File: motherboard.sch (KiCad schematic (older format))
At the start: 90 parts, among them P1 CONN_02X08, U1 STM32F411-LQFP64, U10 74LS125, U11 74LS125, U12 74LS125, U13 74LS125, U14 PCA9517A, U15 PCA9517A, U16 74LS125, U17 74LS125, U2 STM32F411-LQFP64, U3 AP7313, U4 74LS00, U5 74LS125, U6 FM25V20A-G, U7 FM25V20A-G, U8 FM25V20A-G, U9 FM25V20A-G, Y1 32k, Y2 8M(16pF), Y3 32k, Y4 8M(16pF)

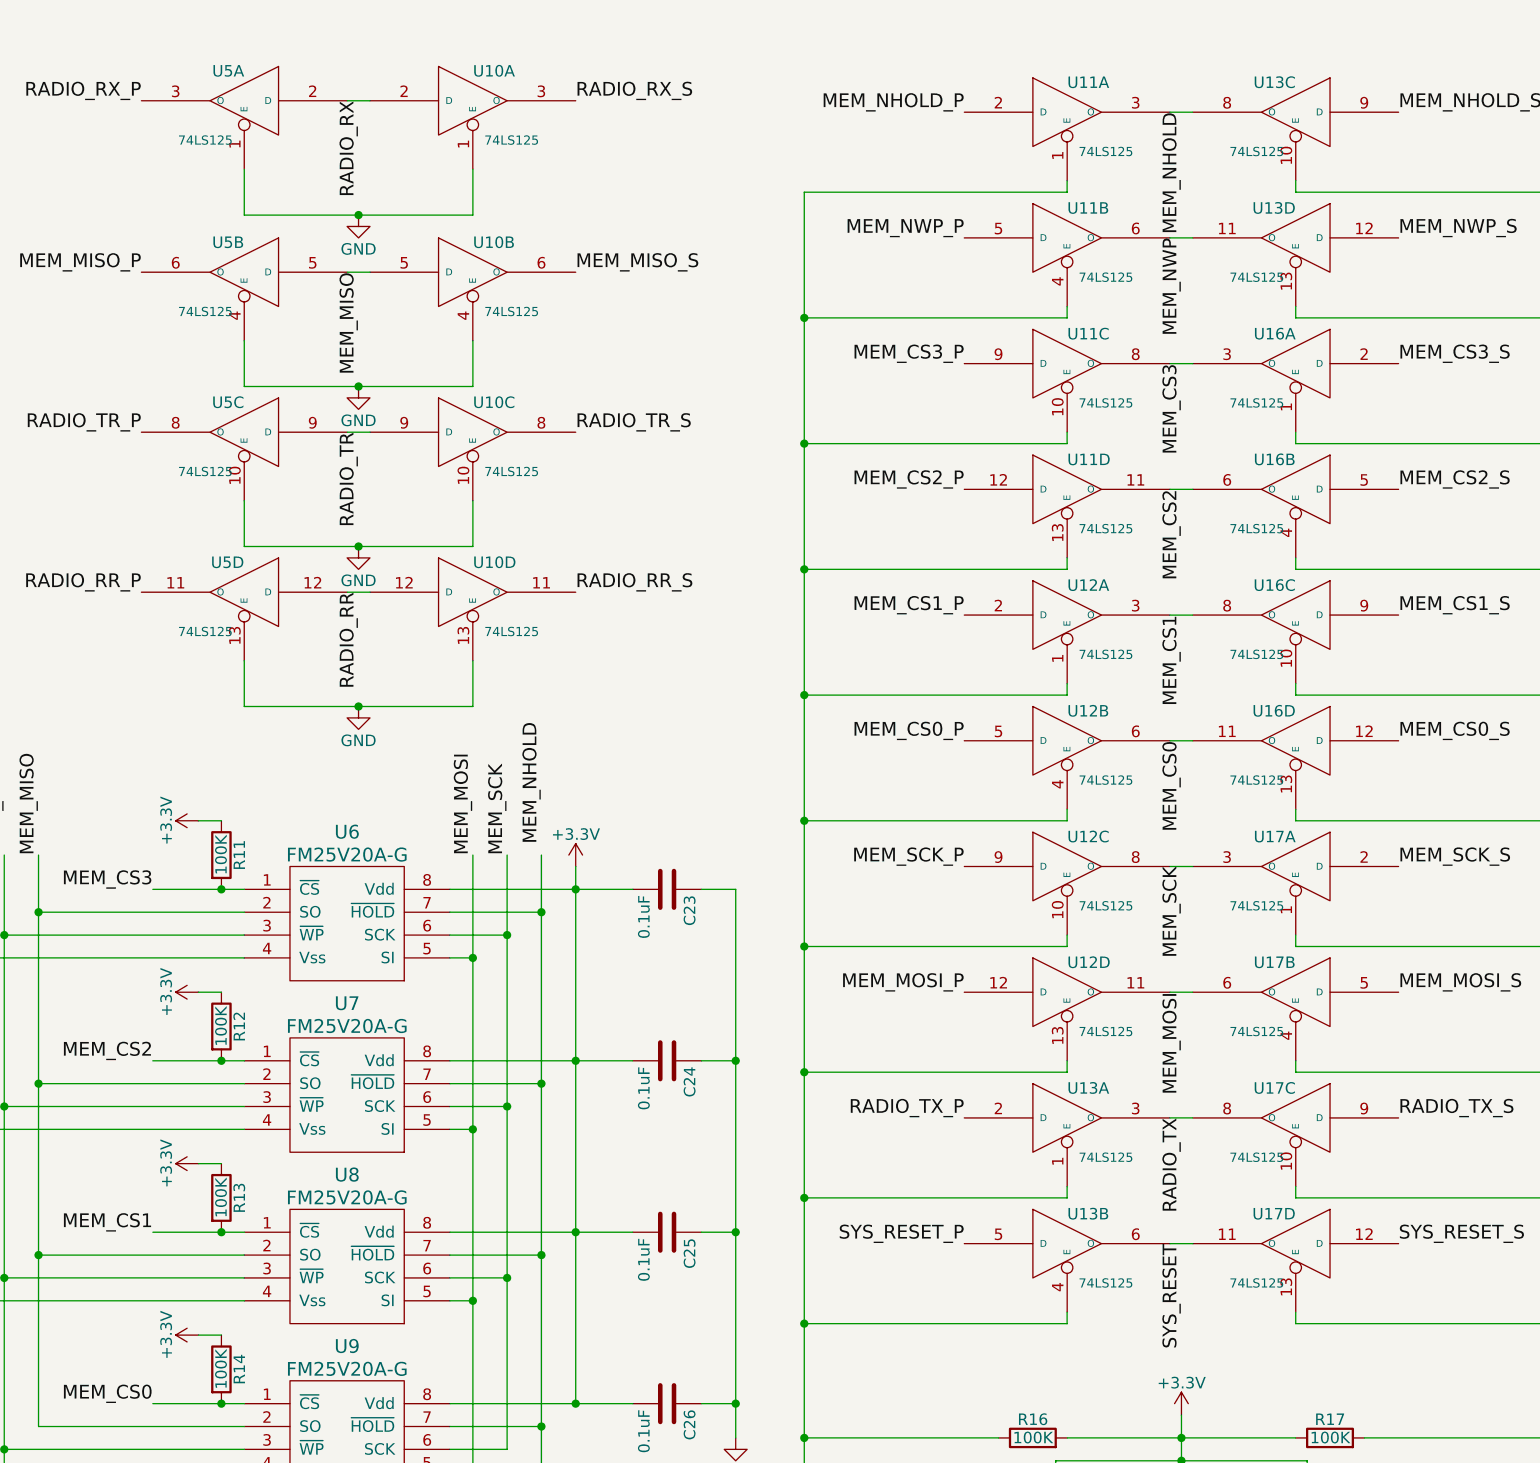
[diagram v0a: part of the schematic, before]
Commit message: Progress in laying out components
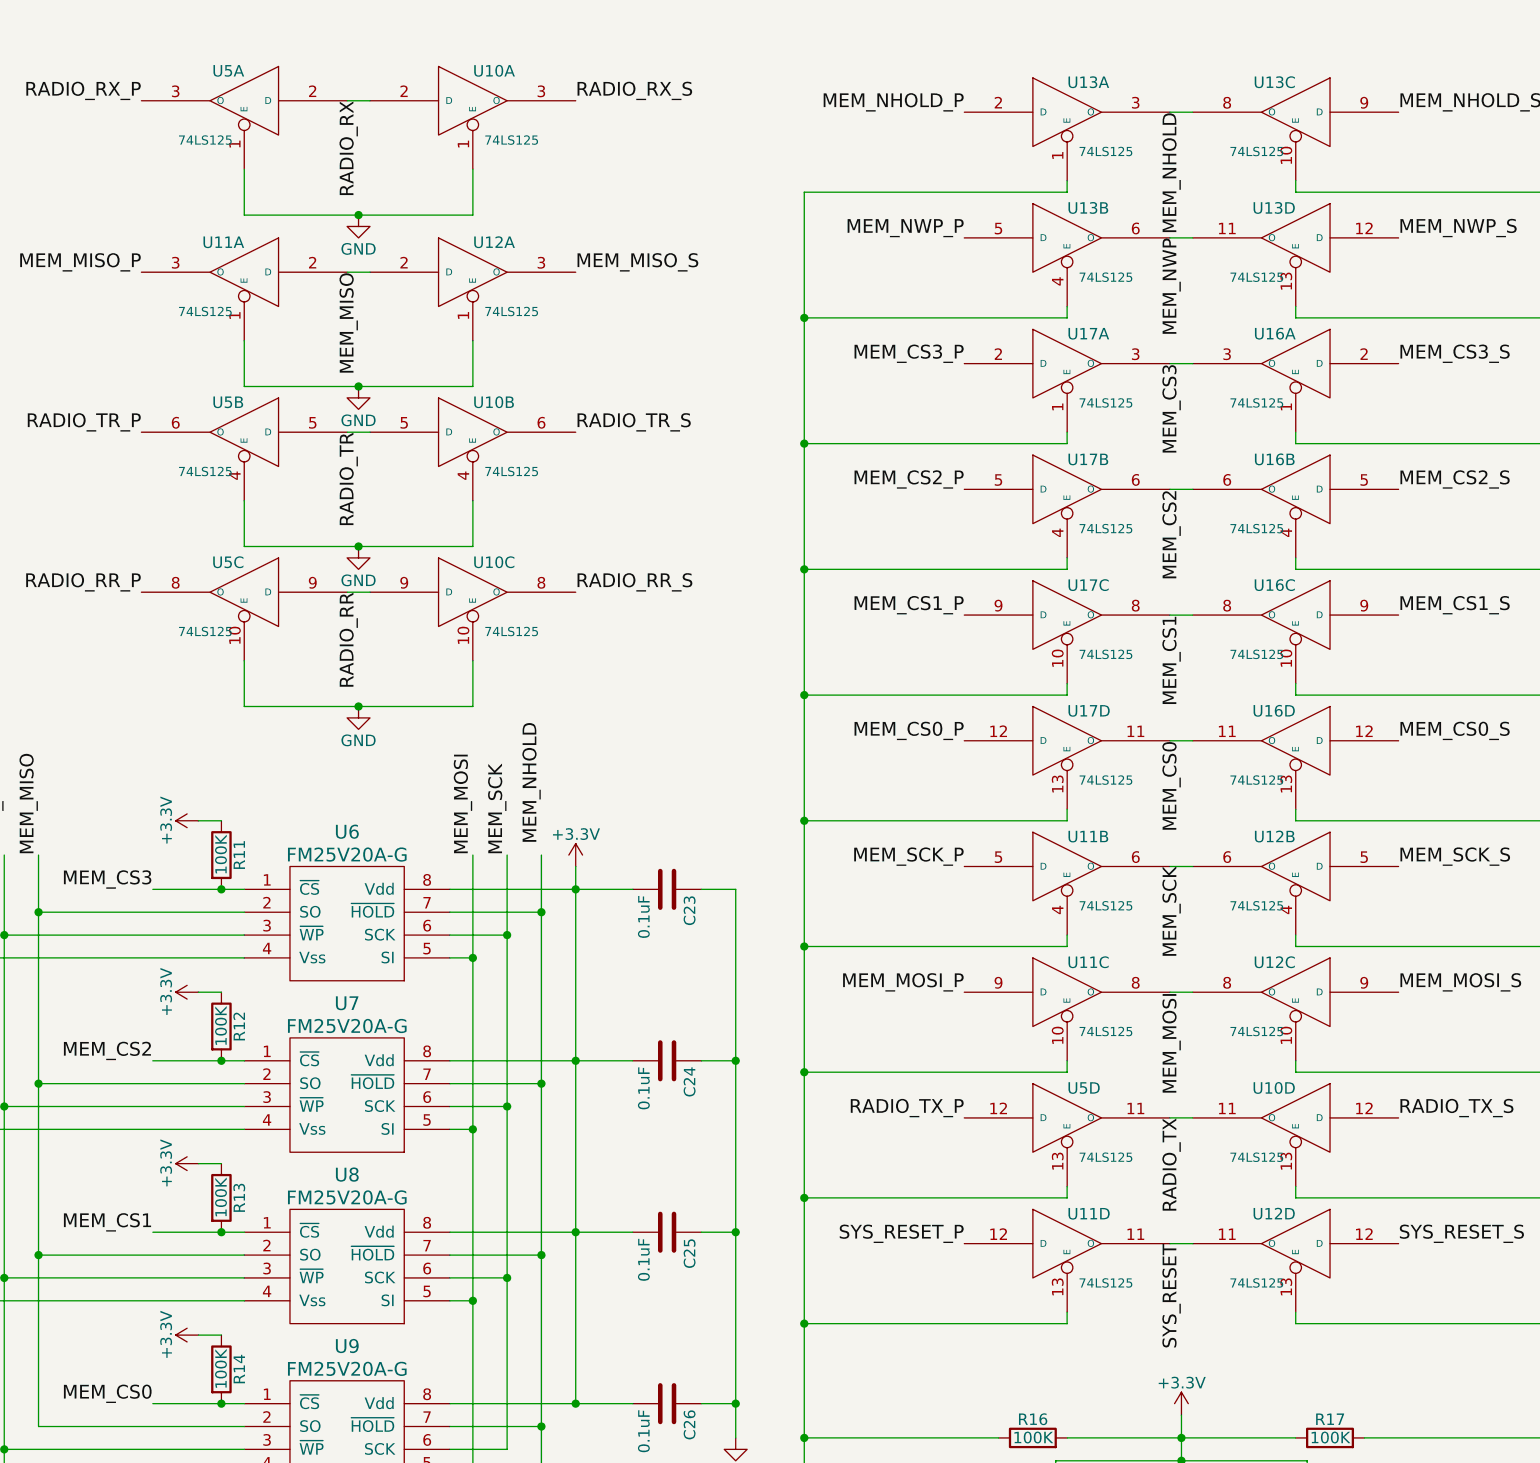
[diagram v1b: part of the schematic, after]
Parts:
- renumbered U17 to U10, U5 to U11, U12 to U11, U13 to U11, U10 to U12, U17 to U12, U11 to U13, U11 to U17, U12 to U17, U13 to U5
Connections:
- net GND: now also U10.10 (E), U10.4 (E), U11.1 (E), U12.1 (E), U5.10 (E), U5.4 (E); no longer U10.10 (E), U10.13 (E), U11.4 (E), U12.4 (E), U5.10 (E), U5.13 (E)
- net MEM_CS0: now also U17.11 (O); no longer U17.6 (O)
- net MEM_CS0_P: now also U17.12 (D); no longer U17.5 (D)
- net MEM_CS1: now also U17.8 (O); no longer U17.3 (O)
- net MEM_CS1_P: now also U17.9 (D); no longer U17.2 (D)
- net MEM_CS2: now also U17.6 (O); no longer U17.11 (O)
- net MEM_CS2_P: now also U17.5 (D); no longer U17.12 (D)
- net MEM_CS3: now also U17.3 (O); no longer U17.8 (O)
- net MEM_CS3_P: now also U17.2 (D); no longer U17.9 (D)
- net MEM_MISO: now also U11.2 (D), U12.2 (D); no longer U11.5 (D), U12.5 (D)
- net MEM_MISO_P: now also U11.3 (O); no longer U11.6 (O)
- net MEM_MISO_S: now also U12.3 (O); no longer U12.6 (O)
- net MEM_MOSI: now also U11.8 (O), U12.8 (O); no longer U11.11 (O), U12.6 (O)
- net MEM_MOSI_P: now also U11.9 (D); no longer U11.12 (D)
- net MEM_MOSI_S: now also U12.9 (D); no longer U12.5 (D)
- net MEM_SCK: now also U11.6 (O), U12.6 (O); no longer U11.8 (O), U12.3 (O)
- net MEM_SCK_P: now also U11.5 (D); no longer U11.9 (D)
- net MEM_SCK_S: now also U12.5 (D); no longer U12.2 (D)
- net NBUFEN_PRI: now also U11.10 (E), U11.13 (E), U11.4 (E), U17.1 (E), U17.10 (E), U17.13 (E), U17.4 (E), U5.13 (E); no longer U11.10 (E), U11.13 (E), U11.4 (E), U17.1 (E), U17.10 (E), U17.13 (E), U17.4 (E), U5.1 (E)
- net NBUFEN_SEC: now also U10.13 (E), U12.10 (E), U12.4 (E); no longer U10.10 (E), U12.1 (E), U12.4 (E)
- net RADIO_RR: now also U10.9 (D), U5.9 (D); no longer U10.12 (D), U5.12 (D)
- net RADIO_RR_P: now also U5.8 (O); no longer U5.11 (O)
- net RADIO_RR_S: now also U10.8 (O); no longer U10.11 (O)
- net RADIO_TR: now also U10.5 (D), U5.5 (D); no longer U10.9 (D), U5.9 (D)
- net RADIO_TR_P: now also U5.6 (O); no longer U5.8 (O)
- net RADIO_TR_S: now also U10.6 (O); no longer U10.8 (O)
- net RADIO_TX: now also U10.11 (O), U5.11 (O); no longer U10.8 (O), U5.3 (O)
- net RADIO_TX_P: now also U5.12 (D); no longer U5.2 (D)
- net RADIO_TX_S: now also U10.12 (D); no longer U10.9 (D)
- net SYS_RESET: now also U11.11 (O); no longer U11.6 (O)
- net SYS_RESET_P: now also U11.12 (D); no longer U11.5 (D)
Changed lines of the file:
@@
 $EndComp
 $Comp
-L 74LS125 U5
-U 2 1 56F0C25F
+L 74LS125 U11
+U 1 1 56F0C25F
 P 8350 1650
-F 0 "U5" H 8350 1750 50  0000 L BNN
+F 0 "U11" H 8350 1750 50  0000 L BNN
 F 1 "74LS125" H 8400 1500 40  0000 L TNN
 F 2 "Housings_SOIC:SOIC-14_3.9x8.7mm_Pitch1.27mm" H 8350 1650 60  0001 C CNN
 F 3 "" H 8350 1650 60  0000 C CNN
-	2    8350 1650
-	-1   0    0    -1
-$EndComp
-$Comp
-L 74LS125 U10
-U 2 1 56F0C346
+	1    8350 1650
+	-1   0    0    -1
+$EndComp
+$Comp
+L 74LS125 U12
+U 1 1 56F0C346
 P 9350 1650
-F 0 "U10" H 9350 1750 50  0000 L BNN
+F 0 "U12" H 9350 1750 50  0000 L BNN
 F 1 "74LS125" H 9400 1500 40  0000 L TNN
 F 2 "Housings_SOIC:SOIC-14_3.9x8.7mm_Pitch1.27mm" H 9350 1650 60  0001 C CNN
 F 3 "" H 9350 1650 60  0000 C CNN
-	2    9350 1650
+	1    9350 1650
 	1    0    0    -1
 $EndComp
@@
 $EndComp
 $Comp
-L 74LS125 U11
+L 74LS125 U13
 U 1 1 56F0DD9C
 P 11950 950
-F 0 "U11" H 11950 1050 50  0000 L BNN
+F 0 "U13" H 11950 1050 50  0000 L BNN
 F 1 "74LS125" H 12000 800 40  0000 L TNN
 F 2 "Housings_SOIC:SOIC-14_3.9x8.7mm_Pitch1.27mm" H 11950 950 60  0001 C CNN
@@
 NYIELD_P
 $Comp
-L 74LS125 U11
+L 74LS125 U13
 U 2 1 56F1CCF5
 P 11950 1500
-F 0 "U11" H 11950 1600 50  0000 L BNN
+F 0 "U13" H 11950 1600 50  0000 L BNN
 F 1 "74LS125" H 12000 1350 40  0000 L TNN
 F 2 "Housings_SOIC:SOIC-14_3.9x8.7mm_Pitch1.27mm" H 11950 1500 60  0001 C CNN
@@
 $EndComp
 $Comp
-L 74LS125 U11
-U 3 1 56F1CE46
+L 74LS125 U17
+U 1 1 56F1CE46
 P 11950 2050
-F 0 "U11" H 11950 2150 50  0000 L BNN
+F 0 "U17" H 11950 2150 50  0000 L BNN
 F 1 "74LS125" H 12000 1900 40  0000 L TNN
 F 2 "Housings_SOIC:SOIC-14_3.9x8.7mm_Pitch1.27mm" H 11950 2050 60  0001 C CNN
 F 3 "" H 11950 2050 60  0000 C CNN
-	3    11950 2050
-	1    0    0    -1
-$EndComp
-$Comp
-L 74LS125 U11
-U 4 1 56F1D346
+	1    11950 2050
+	1    0    0    -1
+$EndComp
+$Comp
+L 74LS125 U17
+U 2 1 56F1D346
 P 11950 2600
-F 0 "U11" H 11950 2700 50  0000 L BNN
+F 0 "U17" H 11950 2700 50  0000 L BNN
 F 1 "74LS125" H 12000 2450 40  0000 L TNN
 F 2 "Housings_SOIC:SOIC-14_3.9x8.7mm_Pitch1.27mm" H 11950 2600 60  0001 C CNN
 F 3 "" H 11950 2600 60  0000 C CNN
-	4    11950 2600
-	1    0    0    -1
-$EndComp
-$Comp
-L 74LS125 U12
-U 1 1 56F1D481
+	2    11950 2600
+	1    0    0    -1
+$EndComp
+$Comp
+L 74LS125 U17
+U 3 1 56F1D481
 P 11950 3150
-F 0 "U12" H 11950 3250 50  0000 L BNN
+F 0 "U17" H 11950 3250 50  0000 L BNN
 F 1 "74LS125" H 12000 3000 40  0000 L TNN
 F 2 "Housings_SOIC:SOIC-14_3.9x8.7mm_Pitch1.27mm" H 11950 3150 60  0001 C CNN
 F 3 "" H 11950 3150 60  0000 C CNN
-	1    11950 3150
-	1    0    0    -1
-$EndComp
-$Comp
-L 74LS125 U12
-U 2 1 56F1D5C5
+	3    11950 3150
+	1    0    0    -1
+$EndComp
+$Comp
+L 74LS125 U17
+U 4 1 56F1D5C5
 P 11950 3700
-F 0 "U12" H 11950 3800 50  0000 L BNN
+F 0 "U17" H 11950 3800 50  0000 L BNN
 F 1 "74LS125" H 12000 3550 40  0000 L TNN
 F 2 "Housings_SOIC:SOIC-14_3.9x8.7mm_Pitch1.27mm" H 11950 3700 60  0001 C CNN
 F 3 "" H 11950 3700 60  0000 C CNN
-	2    11950 3700
-	1    0    0    -1
-$EndComp
-$Comp
-L 74LS125 U12
-U 3 1 56F1DA36
+	4    11950 3700
+	1    0    0    -1
+$EndComp
+$Comp
+L 74LS125 U11
+U 2 1 56F1DA36
 P 11950 4250
-F 0 "U12" H 11950 4350 50  0000 L BNN
+F 0 "U11" H 11950 4350 50  0000 L BNN
 F 1 "74LS125" H 12000 4100 40  0000 L TNN
 F 2 "Housings_SOIC:SOIC-14_3.9x8.7mm_Pitch1.27mm" H 11950 4250 60  0001 C CNN
 F 3 "" H 11950 4250 60  0000 C CNN
-	3    11950 4250
-	1    0    0    -1
-$EndComp
-$Comp
-L 74LS125 U12
-U 4 1 56F1DB80
+	2    11950 4250
+	1    0    0    -1
+$EndComp
+$Comp
+L 74LS125 U11
+U 3 1 56F1DB80
 P 11950 4800
-F 0 "U12" H 11950 4900 50  0000 L BNN
+F 0 "U11" H 11950 4900 50  0000 L BNN
 F 1 "74LS125" H 12000 4650 40  0000 L TNN
 F 2 "Housings_SOIC:SOIC-14_3.9x8.7mm_Pitch1.27mm" H 11950 4800 60  0001 C CNN
 F 3 "" H 11950 4800 60  0000 C CNN
-	4    11950 4800
-	1    0    0    -1
-$EndComp
-$Comp
-L 74LS125 U13
-U 1 1 56F1E3BD
+	3    11950 4800
+	1    0    0    -1
+$EndComp
+$Comp
+L 74LS125 U5
+U 4 1 56F1E3BD
 P 11950 5350
-F 0 "U13" H 11950 5450 50  0000 L BNN
+F 0 "U5" H 11950 5450 50  0000 L BNN
 F 1 "74LS125" H 12000 5200 40  0000 L TNN
 F 2 "Housings_SOIC:SOIC-14_3.9x8.7mm_Pitch1.27mm" H 11950 5350 60  0001 C CNN
 F 3 "" H 11950 5350 60  0000 C CNN
-	1    11950 5350
+	4    11950 5350
 	1    0    0    -1
 $EndComp
@@
 $EndComp
 $Comp
-L 74LS125 U17
-U 1 1 56F39A21
+L 74LS125 U12
+U 2 1 56F39A21
 P 12950 4250
-F 0 "U17" H 12950 4350 50  0000 L BNN
+F 0 "U12" H 12950 4350 50  0000 L BNN
 F 1 "74LS125" H 13000 4100 40  0000 L TNN
 F 2 "Housings_SOIC:SOIC-14_3.9x8.7mm_Pitch1.27mm" H 12950 4250 60  0001 C CNN
 F 3 "" H 12950 4250 60  0000 C CNN
-	1    12950 4250
-	-1   0    0    -1
-$EndComp
-$Comp
-L 74LS125 U17
-U 2 1 56F39B79
+	2    12950 4250
+	-1   0    0    -1
+$EndComp
+$Comp
+L 74LS125 U12
+U 3 1 56F39B79
 P 12950 4800
-F 0 "U17" H 12950 4900 50  0000 L BNN
+F 0 "U12" H 12950 4900 50  0000 L BNN
 F 1 "74LS125" H 13000 4650 40  0000 L TNN
 F 2 "Housings_SOIC:SOIC-14_3.9x8.7mm_Pitch1.27mm" H 12950 4800 60  0001 C CNN
 F 3 "" H 12950 4800 60  0000 C CNN
-	2    12950 4800
-	-1   0    0    -1
-$EndComp
-$Comp
-L 74LS125 U17
-U 3 1 56F3A095
+	3    12950 4800
+	-1   0    0    -1
+$EndComp
+$Comp
+L 74LS125 U10
+U 4 1 56F3A095
 P 12950 5350
-F 0 "U17" H 12950 5450 50  0000 L BNN
+F 0 "U10" H 12950 5450 50  0000 L BNN
 F 1 "74LS125" H 13000 5200 40  0000 L TNN
 F 2 "Housings_SOIC:SOIC-14_3.9x8.7mm_Pitch1.27mm" H 12950 5350 60  0001 C CNN
 F 3 "" H 12950 5350 60  0000 C CNN
-	3    12950 5350
-	-1   0    0    -1
-$EndComp
-$Comp
-L 74LS125 U13
-U 2 1 56F44FCB
+	4    12950 5350
+	-1   0    0    -1
+$EndComp
+$Comp
+L 74LS125 U11
+U 4 1 56F44FCB
 P 11950 5900
-F 0 "U13" H 11950 6000 50  0000 L BNN
+F 0 "U11" H 11950 6000 50  0000 L BNN
 F 1 "74LS125" H 12000 5750 40  0000 L TNN
 F 2 "Housings_SOIC:SOIC-14_3.9x8.7mm_Pitch1.27mm" H 11950 5900 60  0001 C CNN
 F 3 "" H 11950 5900 60  0000 C CNN
-	2    11950 5900
-	1    0    0    -1
-$EndComp
-$Comp
-L 74LS125 U17
+	4    11950 5900
+	1    0    0    -1
+$EndComp
+$Comp
+L 74LS125 U12
 U 4 1 56F45134
 P 12950 5900
-F 0 "U17" H 12950 6000 50  0000 L BNN
+F 0 "U12" H 12950 6000 50  0000 L BNN
 F 1 "74LS125" H 13000 5750 40  0000 L TNN
 F 2 "Housings_SOIC:SOIC-14_3.9x8.7mm_Pitch1.27mm" H 12950 5900 60  0001 C CNN
@@
 $Comp
 L 74LS125 U5
-U 4 1 583EB409
+U 3 1 583EB409
 P 8350 3050
 F 0 "U5" H 8350 3150 50  0000 L BNN
@@
 F 2 "Housings_SOIC:SOIC-14_3.9x8.7mm_Pitch1.27mm" H 8350 3050 60  0001 C CNN
 F 3 "" H 8350 3050 60  0000 C CNN
-	4    8350 3050
+	3    8350 3050
 	-1   0    0    -1
 $EndComp
 $Comp
 L 74LS125 U5
-U 3 1 583EB40F
+U 2 1 583EB40F
 P 8350 2350
 F 0 "U5" H 8350 2450 50  0000 L BNN
@@
 F 2 "Housings_SOIC:SOIC-14_3.9x8.7mm_Pitch1.27mm" H 8350 2350 60  0001 C CNN
 F 3 "" H 8350 2350 60  0000 C CNN
-	3    8350 2350
+	2    8350 2350
 	-1   0    0    -1
 $EndComp
 $Comp
 L 74LS125 U10
-U 3 1 583EB415
+U 2 1 583EB415
 P 9350 2350
 F 0 "U10" H 9350 2450 50  0000 L BNN
@@
 F 2 "Housings_SOIC:SOIC-14_3.9x8.7mm_Pitch1.27mm" H 9350 2350 60  0001 C CNN
 F 3 "" H 9350 2350 60  0000 C CNN
-	3    9350 2350
+	2    9350 2350
 	1    0    0    -1
 $EndComp
 $Comp
 L 74LS125 U10
-U 4 1 583EB41B
+U 3 1 583EB41B
 P 9350 3050
 F 0 "U10" H 9350 3150 50  0000 L BNN
@@
 F 2 "Housings_SOIC:SOIC-14_3.9x8.7mm_Pitch1.27mm" H 9350 3050 60  0001 C CNN
 F 3 "" H 9350 3050 60  0000 C CNN
-	4    9350 3050
-	1    0    0    -1
-$EndComp
+	3    9350 3050
+	1    0    0    -1
+$EndComp
